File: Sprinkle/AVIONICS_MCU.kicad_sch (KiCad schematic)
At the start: 17 parts, among them IC1 ESP32-S3-WROOM-1U-N4R2, IC2 USBLC6-2SC6, J1 Micro_SD_Card, J2 USB_B_Micro, J5 Conn_01x02, SW1 SW_Push, SW2 SW_Push

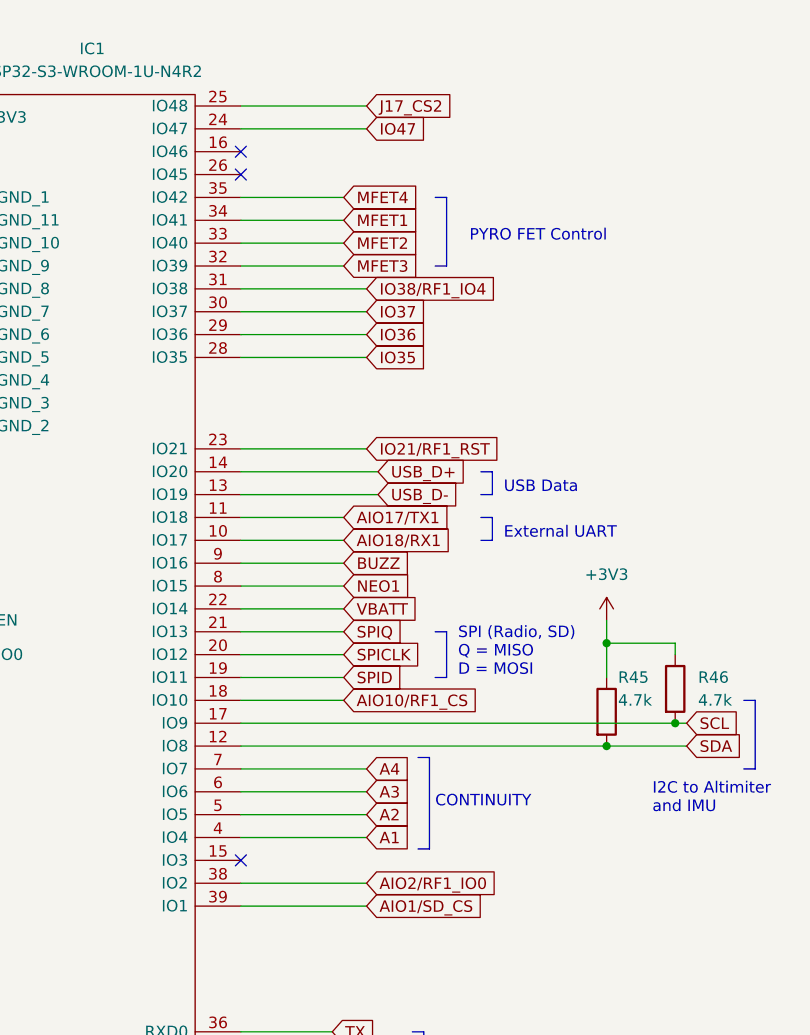
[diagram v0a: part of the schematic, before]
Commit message: Add files via upload
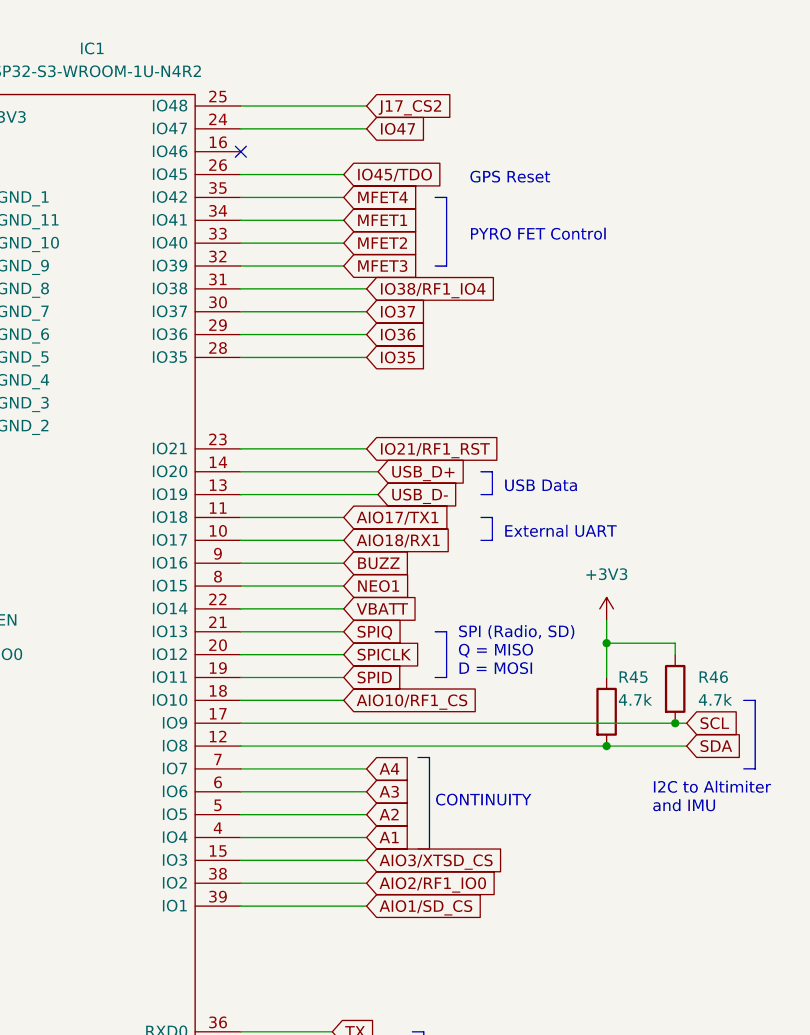
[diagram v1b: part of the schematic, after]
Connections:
- net AIO3/XTSD_CS: now reaches IC1.15 (IO3)
- net IO45/TDO: now reaches IC1.26 (IO45)
- no-connect marks 6 -> 4
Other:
- note added: "GPS Reset"
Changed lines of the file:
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@@
   (junction (at 88.265 44.45) (diameter 0) (color 0 0 0 0)
   )
-  (no_connect (at 220.98 114.3))
   (no_connect (at 69.215 176.53))
   (no_connect (at 83.82 41.91))
   (no_connect (at 83.82 59.69))
   (no_connect (at 220.98 35.56))
-  (no_connect (at 220.98 38.1))
   (wire (pts (xy 184.15 53.34) (xy 187.96 53.34))
     (stroke (width 0) (type default))
@@
     (stroke (width 0) (type default))
   )
+  (wire (pts (xy 220.98 114.3) (xy 234.95 114.3))
+    (stroke (width 0) (type default))
+  )
   (wire (pts (xy 31.75 111.76) (xy 27.94 111.76))
     (stroke (width 0) (type default))
@@
   )
   (wire (pts (xy 184.15 55.88) (xy 187.96 55.88))
+    (stroke (width 0) (type default))
+  )
+  (wire (pts (xy 220.98 38.1) (xy 232.41 38.1))
     (stroke (width 0) (type default))
   )
@@
   (text "USB\n" (at 14.605 97.79 0)
     (effects (font (size 5 5)) (justify left bottom))
+  )
+  (text "GPS Reset\n" (at 246.38 39.37 0)
+    (effects (font (size 1.27 1.27)) (justify left bottom))
   )
   (text "GPS UART" (at 242.57 135.89 0)
@@
     )
   )
+  (global_label "IO45{slash}TDO" (shape input) (at 232.41 38.1 0) (fields_autoplaced)
+    (effects (font (size 1.27 1.27)) (justify left))
+    (property "Intersheetrefs" "${INTERSHEET_REFS}" (at 243.9939 38.1 0)
+      (effects (font (size 1.27 1.27)) (justify left) hide)
+    )
+  )
   (global_label "SCL" (shape input) (at 270.51 99.06 0) (fields_autoplaced)
     (effects (font (size 1.27 1.27)) (justify left))
@@
       (effects (font (size 1.27 1.27)) (justify left) hide)
     )
+  )
+  (global_label "AIO3{slash}XTSD_CS" (shape input) (at 234.95 114.3 0) (fields_autoplaced)
+    (effects (font (size 1.27 1.27)) (justify left))
+    (property "Intersheetrefs" "${INTERSHEET_REFS}" (at 250.8692 114.3 0)
+      (effects (font (size 1.27 1.27)) (justify left) hide)
+    )
